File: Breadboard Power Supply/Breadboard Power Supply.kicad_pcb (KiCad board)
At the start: 2 copper layers, 34.5 x 53.6 mm, 19 parts, among them J1 Conn_01x02_Pin, J2 Conn_01x02_Pin, J3 Conn_01x03_Pin, J4 Conn_01x03_Pin, J5 Screw_Terminal_01x02, J6 Barrel_Jack_Switch, J7 Screw_Terminal_01x02, U1 LM7805, U2 LM317

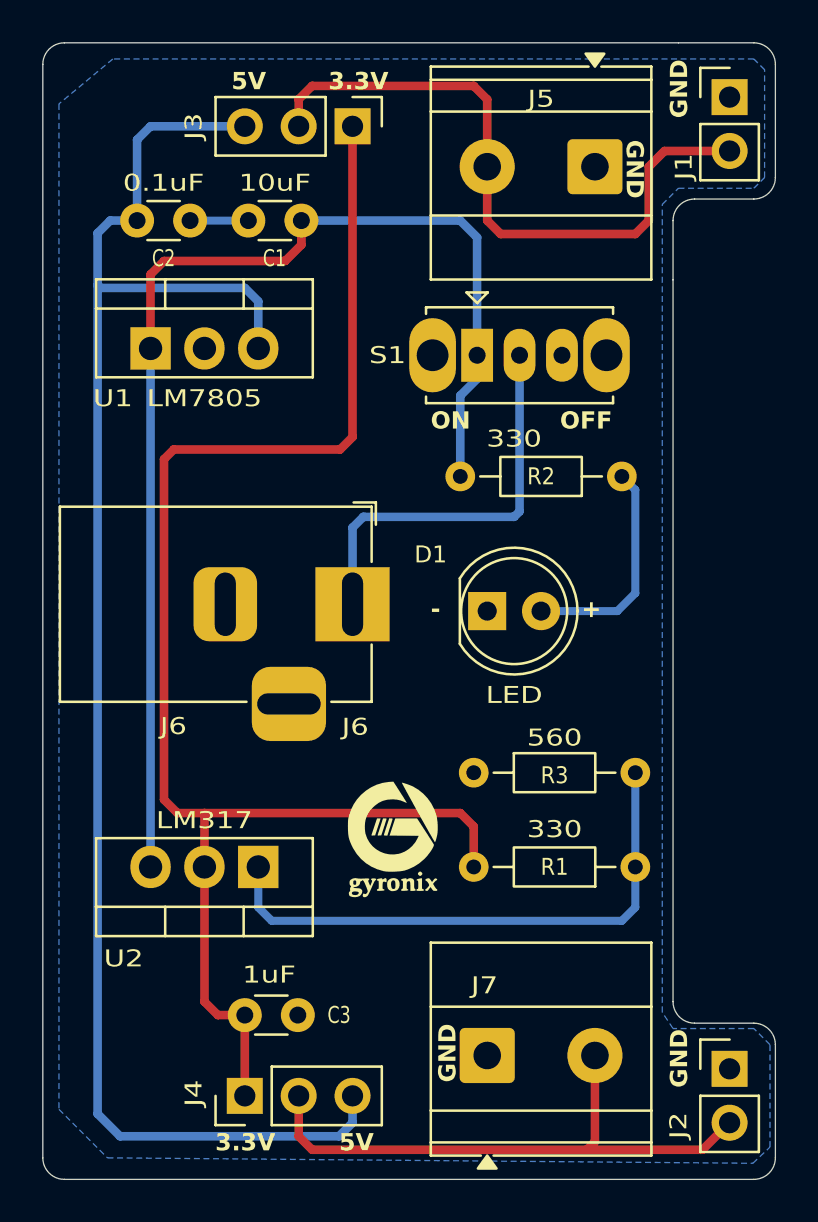
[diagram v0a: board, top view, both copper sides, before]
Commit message: update
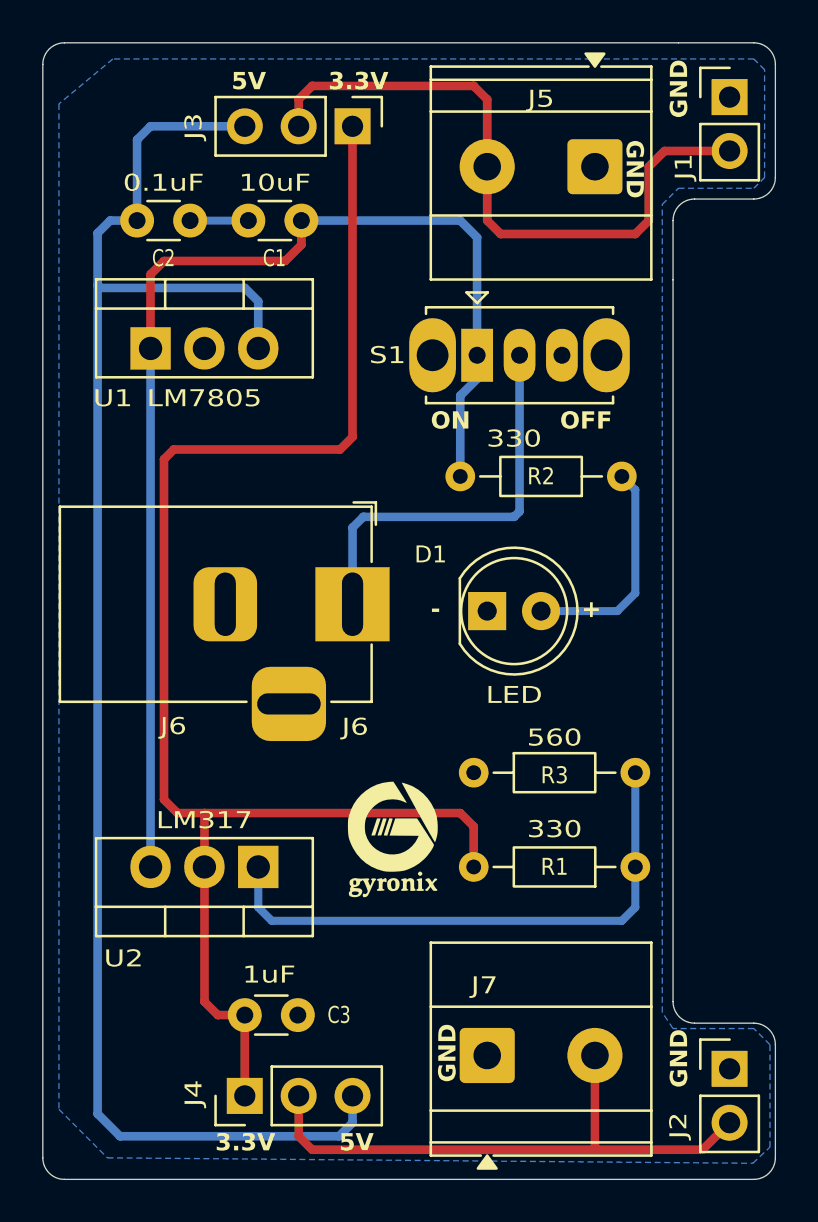
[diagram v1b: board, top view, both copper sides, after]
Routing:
- net GND: track 3.42 -> 2.80 mm
